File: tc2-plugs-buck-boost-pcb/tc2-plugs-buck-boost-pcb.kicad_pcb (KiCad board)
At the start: 6 copper layers, 65 x 19.5 mm, 68 parts, among them J201 JCON_M16_04Pin, J202 JCON_M16_2+4Pin, J203 Conn_02x06_Odd_Even, Q201 Q_PMOS_GSD, Q202 Q_PMOS_GSD, Q203 AO3400A, U201 TPS63070RNMR, U202 TPS63071

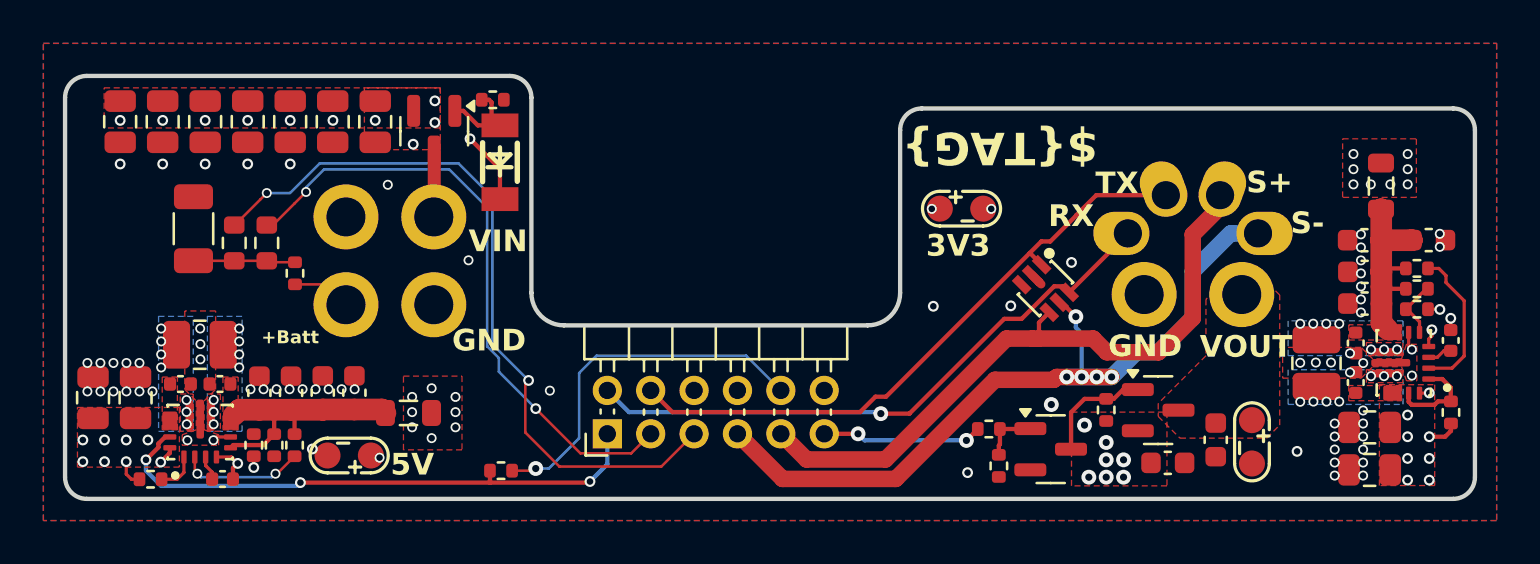
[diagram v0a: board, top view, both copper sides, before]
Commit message: version v0.7.1
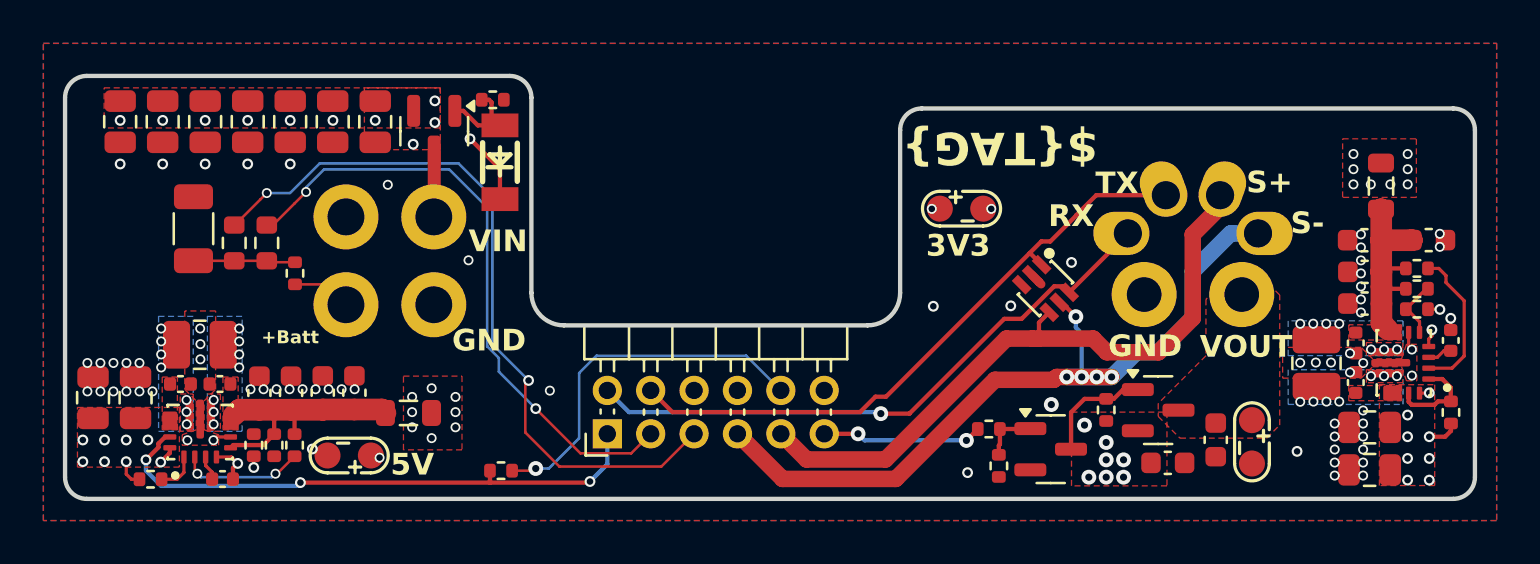
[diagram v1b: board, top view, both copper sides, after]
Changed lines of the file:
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@@
 			(at -2.25 1.58 90)
 			(size 3 3)
-			(drill 1.8)
+			(drill 1.6)
 			(layers "*.Cu" "*.Mask")
 			(remove_unused_layers no)
@@
 			(pintype "passive")
 			(clearance 0.3)
-			(thermal_gap 1)
+			(thermal_gap 0.7)
 		)
 		(pad "2" thru_hole oval
@@
 			(at 2.25 1.58 90)
 			(size 3 3)
-			(drill 1.8)
+			(drill 1.6)
 			(layers "*.Cu" "*.Mask")
 			(remove_unused_layers no)
@@
 			(at -2.025 2.025 90)
 			(size 3 3)
-			(drill 1.8)
+			(drill 1.7)
 			(layers "*.Cu" "*.Mask")
 			(remove_unused_layers no)
 			(net 1 "GND")
 			(pintype "passive")
-			(thermal_gap 1.2)
+			(thermal_gap 0.7)
 		)
 		(pad "2" thru_hole circle
 			(at 2.025 2.025 90)
 			(size 3 3)
-			(drill 1.8)
+			(drill 1.7)
 			(layers "*.Cu" "*.Mask")
 			(remove_unused_layers no)
@@
 			(at 2.025 -2.025 90)
 			(size 3 3)
-			(drill 1.8)
+			(drill 1.7)
 			(layers "*.Cu" "*.Mask")
 			(remove_unused_layers no)
@@
 			(at -2.025 -2.025 90)
 			(size 3 3)
-			(drill 1.8)
+			(drill 1.7)
 			(layers "*.Cu" "*.Mask")
 			(remove_unused_layers no)
